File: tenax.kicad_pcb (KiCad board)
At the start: 2 copper layers, 249 x 99.5 mm, 54 parts, among them J1 AudioJack4, J2 AudioJack4, SW1 SW_SPST, SW10 SW_SPST, SW11 SW_SPST, SW12 SW_SPST, SW13 SW_SPST, SW14 SW_SPST, SW15 SW_SPST, SW16 SW_SPST, SW17 SW_SPST, SW18 SW_SPST, SW19 SW_SPST, SW2 SW_SPST, SW20 SW_SPST, SW21 SW_SPST, SW22 SW_SPST, SW23 SW_SPST, SW24 SW_SPST, SW25 SW_SPST, SW26 SW_SPST, SW27 SW_SPST, SW28 SW_SPST, SW29 SW_SPST, SW3 SW_SPST, SW30 SW_SPST, SW31 SW_SPST, SW32 SW_SPST, SW33 SW_SPST, SW34 SW_SPST, SW35 SW_SPST, SW36 SW_SPST, SW4 SW_SPST, SW5 SW_SPST, SW6 SW_SPST, SW7 SW_SPST, SW8 SW_SPST, SW9 SW_SPST, U1 YAAJ_WeAct_BlackPill_Part_Like, U2 YAAJ_WeAct_BlackPill_Part_Like

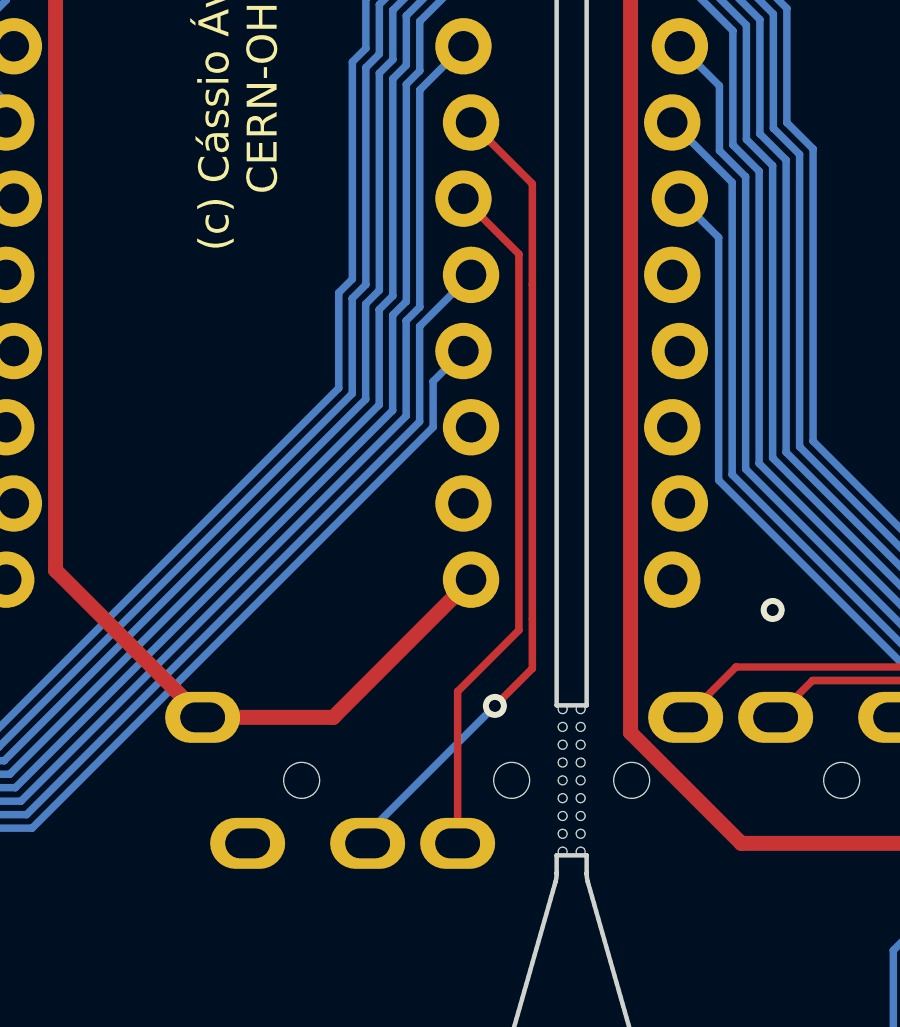
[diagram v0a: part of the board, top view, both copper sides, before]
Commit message: teardrops
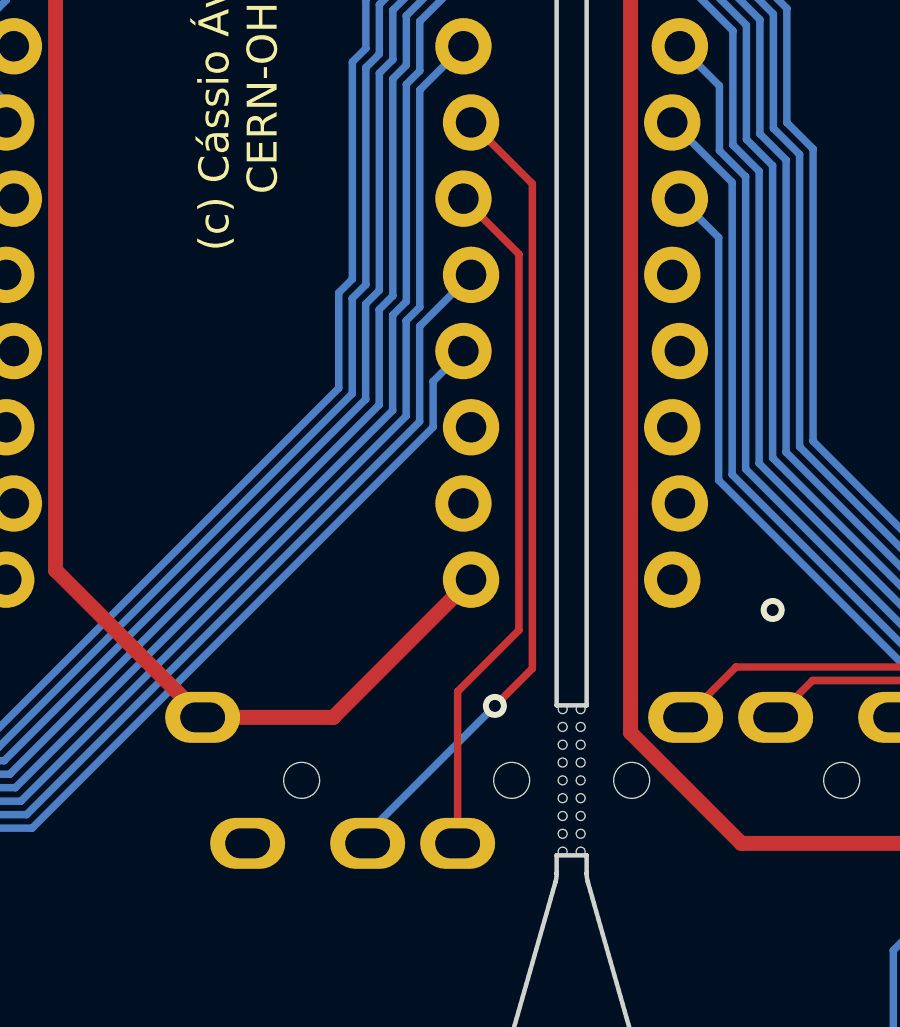
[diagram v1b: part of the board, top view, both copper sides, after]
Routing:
- net TX_l: track 27.6 -> 26.8 mm
